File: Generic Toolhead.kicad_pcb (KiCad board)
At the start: 2 copper layers, 77 parts, among them Q1 LND150, Q2 LND150, Q3 LND150, Q4 LND150, U1 ADXL345, U2 RP2040, U3 TMC2209

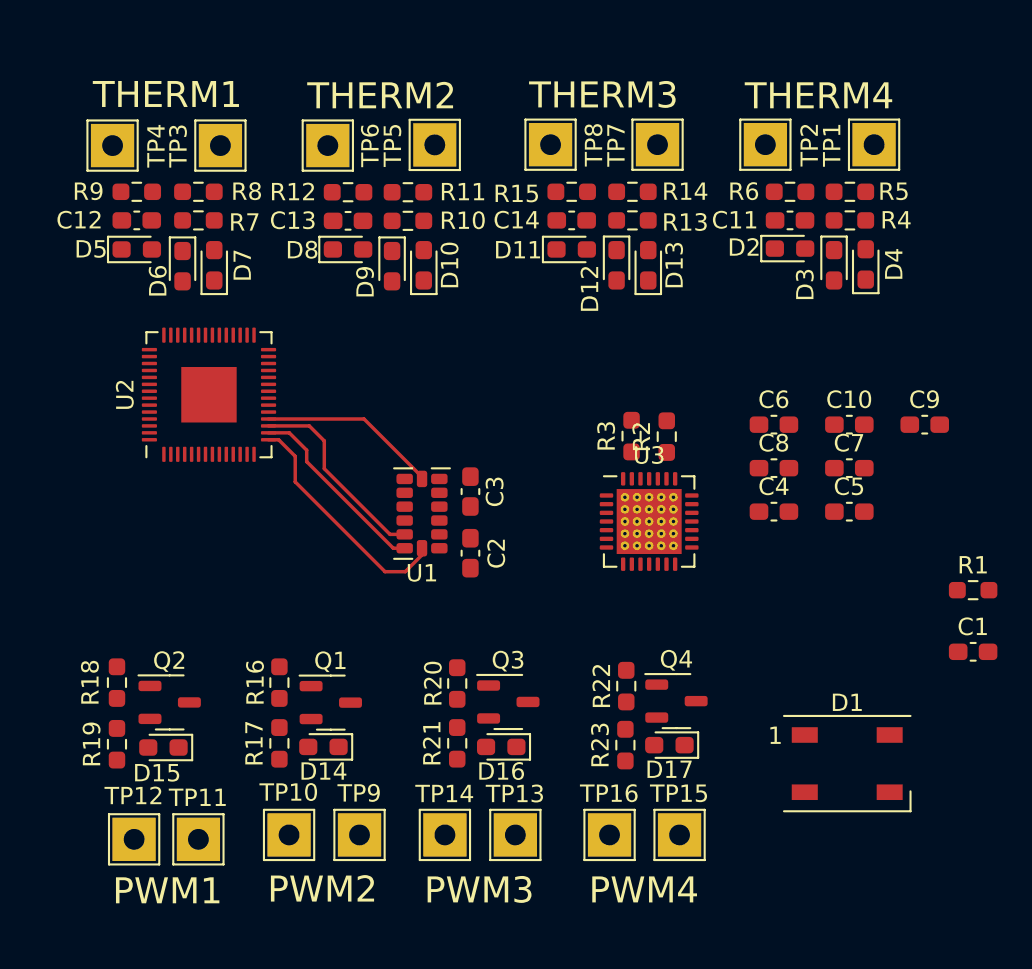
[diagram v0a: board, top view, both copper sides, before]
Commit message: More big changes. Almost entirely done.
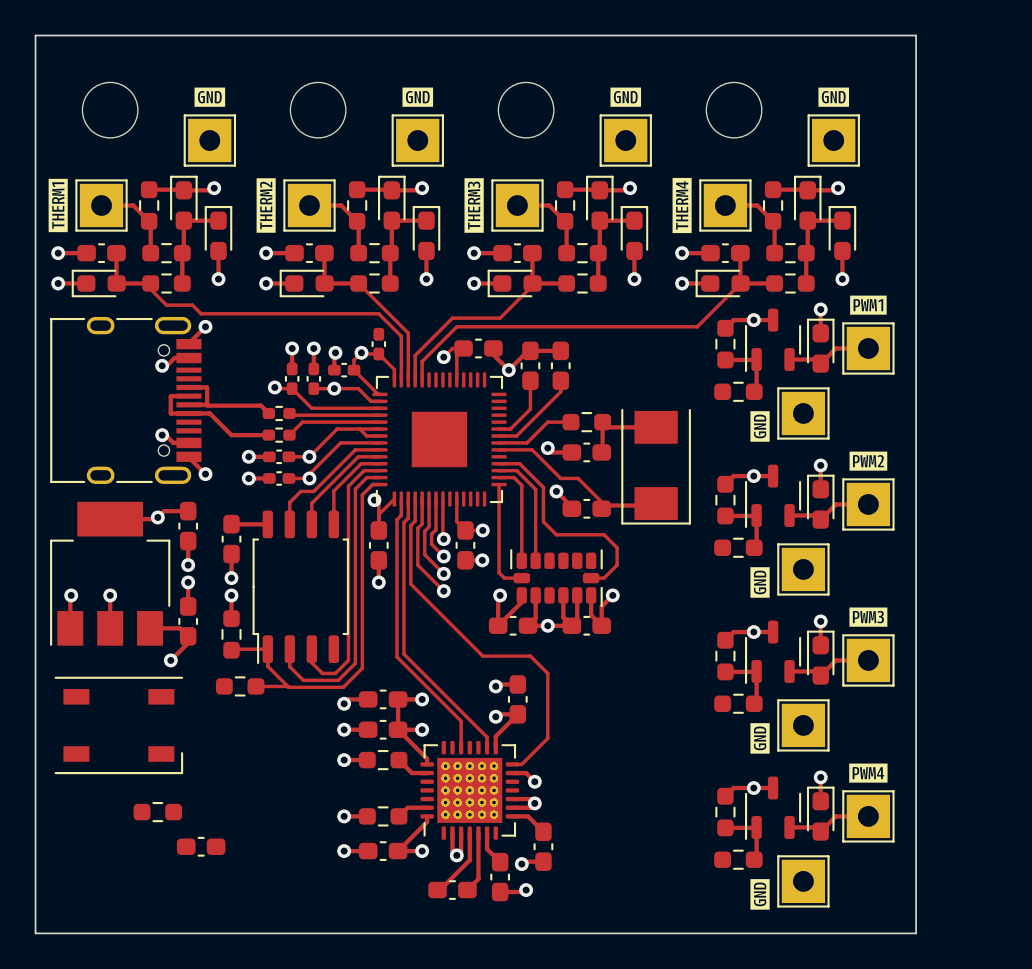
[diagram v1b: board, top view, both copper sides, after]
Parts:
- added C15: 100n, Capacitor_SMD:C_0603_1608Metric_Pad1.08x0.95mm_HandSolder, F.Cu at (40.8, 31.2)
- added C16: 100n, Capacitor_SMD:C_0402_1005Metric_Pad0.74x0.62mm_HandSolder, F.Cu at (26.2, 37.8)
- added C17: 1u, Capacitor_SMD:C_0402_1005Metric_Pad0.74x0.62mm_HandSolder, F.Cu at (27.0, 32.0)
- added C18: 100n, Capacitor_SMD:C_0402_1005Metric_Pad0.74x0.62mm_HandSolder, F.Cu at (32.0, 30.0)
- added C19: 100n, Capacitor_SMD:C_0603_1608Metric_Pad1.08x0.95mm_HandSolder, F.Cu at (42.5, 31.2)
- added C20: 1u, Capacitor_SMD:C_0402_1005Metric_Pad0.74x0.62mm_HandSolder, F.Cu at (28.2, 32.0)
- added C21: 100n, Capacitor_SMD:C_0603_1608Metric_Pad1.08x0.95mm_HandSolder, F.Cu at (37.8, 30.2)
- added C22: 100n, Capacitor_SMD:C_0402_1005Metric_Pad0.74x0.62mm_HandSolder, F.Cu at (26.2, 36.5)
- added C23: 100n, Capacitor_SMD:C_0603_1608Metric_Pad1.08x0.95mm_HandSolder, F.Cu at (37.0, 41.6)
- added C24: 100n, Capacitor_SMD:C_0402_1005Metric_Pad0.74x0.62mm_HandSolder, F.Cu at (30.0, 31.5)
- added C25: 100n, Capacitor_SMD:C_0603_1608Metric_Pad1.08x0.95mm_HandSolder, F.Cu at (32.0, 41.6)
- added C26: 10u, Capacitor_SMD:C_0603_1608Metric_Pad1.08x0.95mm_HandSolder, F.Cu at (21.0, 46.0)
- added C27: 10u, Capacitor_SMD:C_0603_1608Metric_Pad1.08x0.95mm_HandSolder, F.Cu at (21.0, 40.5)
- added C28: 100n, Capacitor_SMD:C_0603_1608Metric_Pad1.08x0.95mm_HandSolder, F.Cu at (23.5, 41.2)
- added C29: 27p, Capacitor_SMD:C_0603_1608Metric_Pad1.08x0.95mm_HandSolder, F.Cu at (44.0, 39.5)
- added C30: 27p, Capacitor_SMD:C_0603_1608Metric_Pad1.08x0.95mm_HandSolder, F.Cu at (44.0, 36.2)
- added J2: USB_C_Receptacle_USB2.0, Connector_USB:USB_C_Receptacle_HRO_TYPE-C-31-M-12, F.Cu at (17.0, 33.2)
- added R24: 27_4, Resistor_SMD:R_0402_1005Metric_Pad0.72x0.64mm_HandSolder, F.Cu at (26.2, 35.2)
- added R25: 27_4, Resistor_SMD:R_0402_1005Metric_Pad0.72x0.64mm_HandSolder, F.Cu at (26.2, 34.0)
- added R26: 1k, Resistor_SMD:R_0603_1608Metric_Pad0.98x0.95mm_HandSolder, F.Cu at (24.0, 49.8)
- added R27: 10k, Resistor_SMD:R_0603_1608Metric_Pad0.98x0.95mm_HandSolder, F.Cu at (23.5, 46.8)
- added R28: 1k, Resistor_SMD:R_0603_1608Metric_Pad0.98x0.95mm_HandSolder, F.Cu at (44.0, 34.5)
- added REF**: MountingHole_3.2mm_M3, MountingHole:MountingHole_3.2mm_M3, F.Cu at (16.5, 16.5)
- added REF**: MountingHole_3.2mm_M3, MountingHole:MountingHole_3.2mm_M3, F.Cu at (40.5, 16.5)
- added REF**: MountingHole_3.2mm_M3, MountingHole:MountingHole_3.2mm_M3, F.Cu at (28.5, 16.5)
- added REF**: MountingHole_3.2mm_M3, MountingHole:MountingHole_3.2mm_M3, F.Cu at (52.5, 16.5)
- added U4: AP1117-33, Package_TO_SOT_SMD:SOT-223-3_TabPin2, F.Cu at (16.5, 43.2)
- added U5: W25Q128JVS, Package_SO:SOIC-8_5.23x5.23mm_P1.27mm, F.Cu at (27.5, 44.0)
- added Y1: Crystal, Crystal:Crystal_SMD_0603-2Pin_6.0x3.5mm, F.Cu at (48.0, 37.0)
- added kibuzzard-64D9AE25: G***, kibuzzard-64D9AE25, F.Cu at (13.5, 22.0)
- added kibuzzard-64D9AE55: G***, kibuzzard-64D9AE55, F.Cu at (25.5, 22.0)
- added kibuzzard-64D9AE6A: G***, kibuzzard-64D9AE6A, F.Cu at (37.5, 22.0)
- added kibuzzard-64D9AE78: G***, kibuzzard-64D9AE78, F.Cu at (49.5, 22.0)
- added kibuzzard-64D9AF4B: G***, kibuzzard-64D9AF4B, F.Cu at (58.2, 15.8)
- added kibuzzard-64D9AF4B: G***, kibuzzard-64D9AF4B, F.Cu at (46.2, 15.8)
- added kibuzzard-64D9AF4B: G***, kibuzzard-64D9AF4B, F.Cu at (22.2, 15.8)
- added kibuzzard-64D9AF4B: G***, kibuzzard-64D9AF4B, F.Cu at (34.2, 15.8)
- added kibuzzard-64D9D5AA: G***, kibuzzard-64D9D5AA, F.Cu at (60.2, 27.8)
- added kibuzzard-64D9D5C0: G***, kibuzzard-64D9D5C0, F.Cu at (60.2, 36.8)
- added kibuzzard-64D9D5CE: G***, kibuzzard-64D9D5CE, F.Cu at (60.2, 45.8)
- added kibuzzard-64D9D5DA: G***, kibuzzard-64D9D5DA, F.Cu at (60.2, 54.8)
- added kibuzzard-64D9D5F2: G***, kibuzzard-64D9D5F2, F.Cu at (54.0, 52.8)
- added kibuzzard-64D9D5F2: G***, kibuzzard-64D9D5F2, F.Cu at (54.0, 61.8)
- added kibuzzard-64D9D5F2: G***, kibuzzard-64D9D5F2, F.Cu at (54.0, 43.8)
- added kibuzzard-64D9D5F2: G***, kibuzzard-64D9D5F2, F.Cu at (54.0, 34.8)
- moved R1 48.8 mm to (19.2, 57.0)
- moved C1 45.9 mm to (21.8, 59.0)
- moved TP1 44.7 mm to (16.0, 22.0)
- moved TP11 43.2 mm to (60.2, 39.2), turned to 90 degrees
- moved D1 42.1 mm to (17.0, 52.0)
- moved TP12 41.6 mm to (56.5, 43.0), turned to 90 degrees
- moved TP9 40.6 mm to (60.2, 30.2), turned to 90 degrees
- moved D15 40.4 mm to (57.5, 39.2), turned to -90 degrees
- moved D2 39.8 mm to (16.0, 26.5)
- moved C11 39.8 mm to (16.0, 24.8)
- moved R4 39.6 mm to (19.8, 26.5)
- moved R5 39.6 mm to (19.8, 24.8)
- moved D4 39.5 mm to (20.8, 22.0), turned to -90 degrees
- moved TP10 38.4 mm to (56.5, 34.0), turned to 90 degrees
- moved C9 38.3 mm to (36.2, 61.5)
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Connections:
- net /MCU_ADXL_CS renamed /ADXL/CS
- net /MCU_ADXL_SCL renamed /ADXL/SCL
- net /MCU_ADXL_SDA renamed /ADXL/SDA
- net /MCU_ADXL_SDO renamed /ADXL/SDO
- U1 pad 8: /MCU_ADXL_INT1 -> unconnected-(U1-Pad8)
- U1 pad 9: /MCU_ADXL_INT2 -> unconnected-(U1-Pad9)
- U2 pad 1: Net-(U2-Pad1) -> +3V3
- U2 pad 10: Net-(U2-Pad1) -> +3V3
- U2 pad 20: unconnected-(U2-Pad20) -> /Oscillator/XIN
- U2 pad 21: unconnected-(U2-Pad21) -> /Oscillator/XOUT
- U2 pad 22: Net-(U2-Pad1) -> +3V3
- U2 pad 23: Net-(U2-Pad23) -> +1V1
- U2 pad 33: Net-(U2-Pad1) -> +3V3
- U2 pad 42: Net-(U2-Pad1) -> +3V3
- U2 pad 43: unconnected-(U2-Pad43) -> +3V3
- U2 pad 44: unconnected-(U2-Pad44) -> +3V3
- U2 pad 45: unconnected-(U2-Pad45) -> +1V1
- U2 pad 46: /USB_DM -> Net-(R25-Pad1)
- U2 pad 47: /USB_DP -> Net-(R24-Pad2)
- U2 pad 48: unconnected-(U2-Pad48) -> +3V3
- U2 pad 49: Net-(U2-Pad1) -> +3V3
- U2 pad 50: Net-(U2-Pad23) -> +1V1
- U2 pad 51: unconnected-(U2-Pad51) -> /QSPI_SD3
- U2 pad 52: unconnected-(U2-Pad52) -> /QSPI_SCLK
- U2 pad 53: unconnected-(U2-Pad53) -> /QSPI_SD0
- U2 pad 54: unconnected-(U2-Pad54) -> /QSPI_SD2
- U2 pad 55: unconnected-(U2-Pad55) -> /QSPI_SD1
- U2 pad 56: unconnected-(U2-Pad56) -> /QSPI_SS
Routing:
- net GND: track 0.00 -> 81.1 mm, vias 0 -> 43
- net +3V3: track 0.00 -> 70.3 mm, vias 0 -> 16
- net /Thermistor3/TH_MCU: track 0.00 -> 25.0 mm
- net /QSPI_SS: track 0.00 -> 22.7 mm
- net /Thermistor/TH_MCU: track 0.00 -> 22.2 mm
- net /Motor Driver/UART: track 0.00 -> 21.5 mm
- net +24V: track 0.00 -> 18.3 mm, vias 0 -> 8
- net /QSPI_SD1: track 0.00 -> 17.3 mm
- net +1V1: track 0.00 -> 16.7 mm, vias 0 -> 2
- net /Motor Driver/STEP: track 0.00 -> 16.4 mm
- net /Motor Driver/DIR: track 0.00 -> 16.0 mm
- net /QSPI_SD2: track 0.00 -> 15.7 mm
- net /Thermistor2/TH_MCU: track 0.00 -> 13.7 mm
- net /Oscillator/XIN: track 0.00 -> 10.8 mm
- net /Thermistor1/TH_MCU: track 0.00 -> 10.5 mm
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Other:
- board outline added: 50.8 x 51.8 mm
- board text removed: "PWM1"
- board text removed: "PWM2"
- board text removed: "PWM3"
- board text removed: "PWM4"
- board text removed: "THERM1"
- board text removed: "THERM2"
- board text removed: "THERM3"
- board text removed: "THERM4"
